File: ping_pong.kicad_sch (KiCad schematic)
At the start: 56 parts, among them J101 5V_IN, J102 AMMETER-, J103 GND_IN, J104 STEPPER_OUT1, J105 ENABLE, J106 STEP1, J107 DIR1, J108 AMMETER+, J109 STEP2, J110 DIR2, J111 STEPPER_OUT2, J112 12V_IN, J113 STEP3, J114 DIR3, J115 STEPPER_OUT3, J117 STEP4, J118 DIR4, J119 STEPPER_OUT4, J120 6V_for_Hbridge, J121 5V_for_ultrasonic1, J122 5V_for_ultrasonic2, J123 5V_for_ultrasonic3, J124 5V_for_ultrasonic4, J125 GND_for_ultrasonic1, J126 GND_for_ultrasonic2, J127 GND_for_ultrasonic3, J128 GND_for_ultrasonic4, J129 5V_for_pixycam, J130 GND_for_Hbridge, J131 3.3V_IN, J132 GND_for_xbee, J133 GND_for_pixycam, J134 GND_backup1, J135 GND_backup2, J138 5V_backup1, J139 5V_backup2, J140 5V_backup3, J141 5V_backup4, J142 3.3V_for_xbee, J143 3.3V_backup1, J144 3.3V_backup2, J145 5V_SERVO1, J146 5V_SERVO2, J147 GND_SERVO1, J148 GND_SERVO1

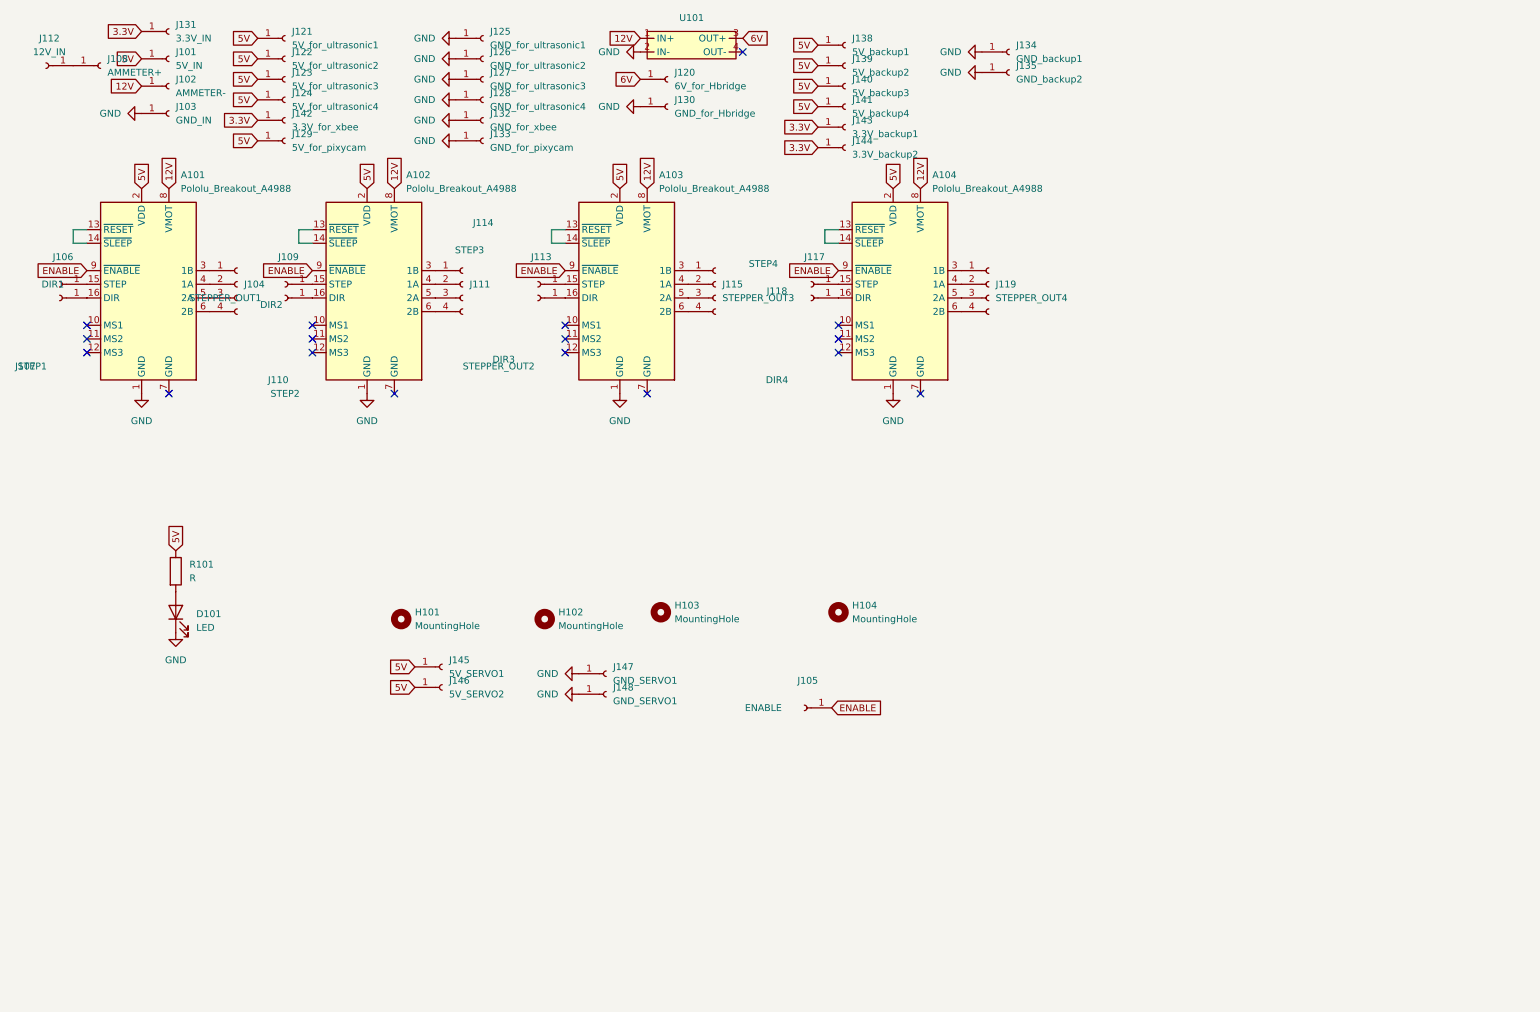
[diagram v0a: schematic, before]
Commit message: checkpoint
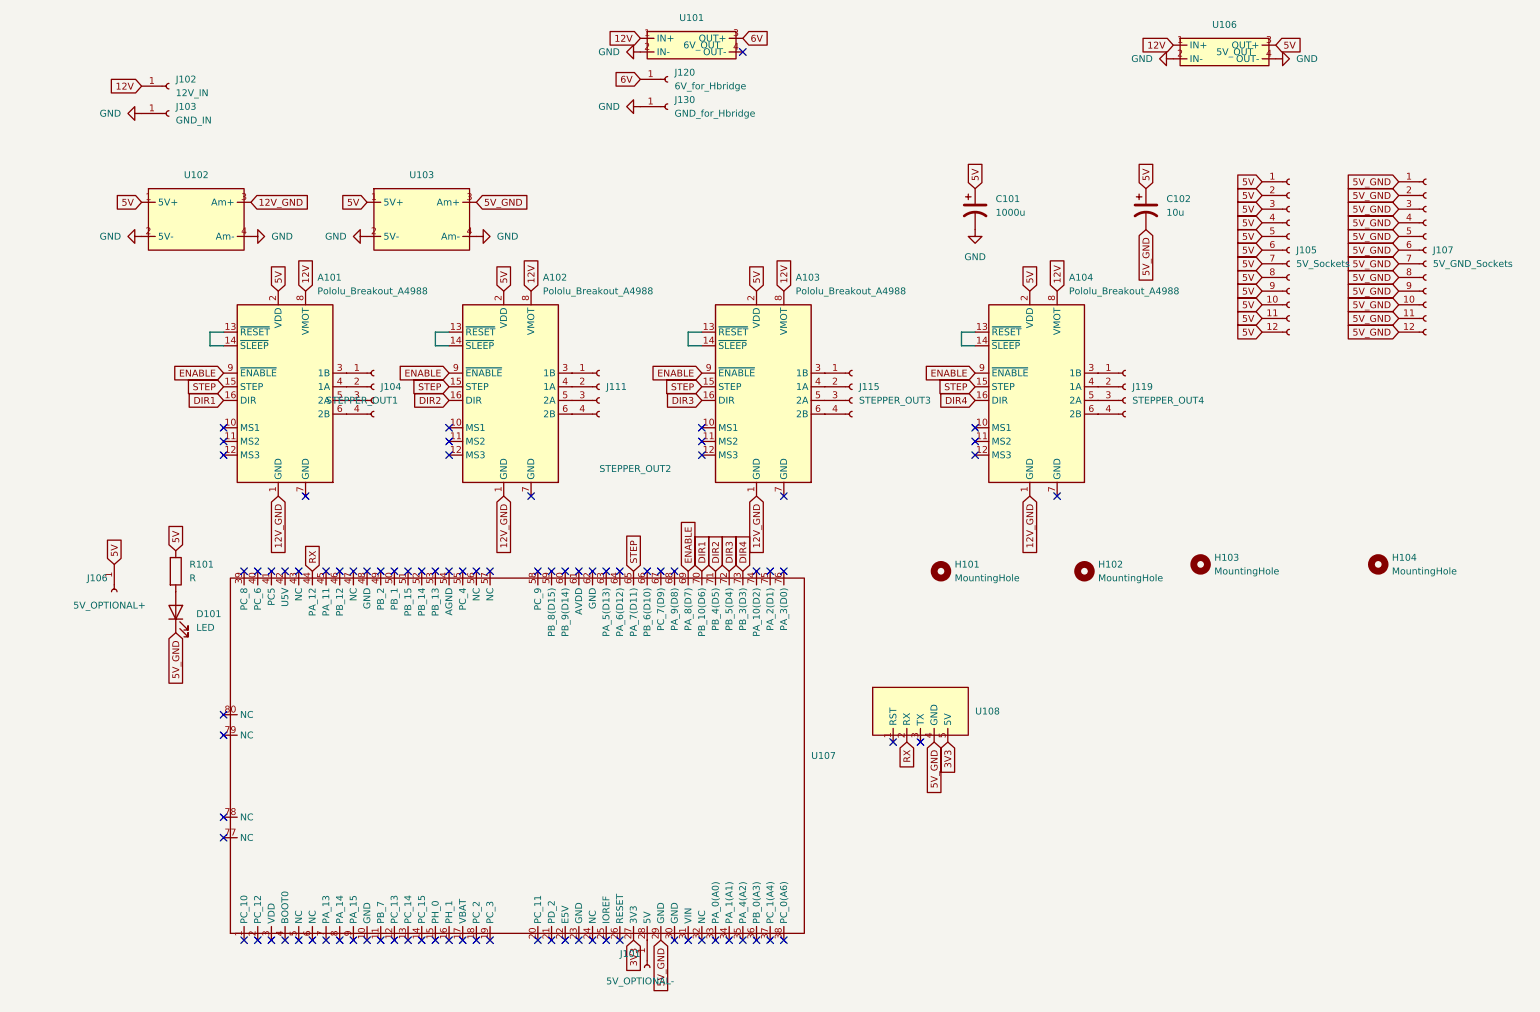
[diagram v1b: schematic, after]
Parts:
- removed J105: ENABLE, MyPinSocket:MyPinSocket, symbol Connector:Conn_01x01_Socket
- removed J107: DIR1, MyPinSocket:MyPinSocket, symbol Connector:Conn_01x01_Socket
- removed J108: AMMETER+, MyPinSocket:MyPinSocket, symbol Connector:Conn_01x01_Socket
- removed J109: STEP2, MyPinSocket:MyPinSocket, symbol Connector:Conn_01x01_Socket
- removed J110: DIR2, MyPinSocket:MyPinSocket, symbol Connector:Conn_01x01_Socket
- removed J112: 12V_IN, MyPinSocket:MyPinSocket, symbol Connector:Conn_01x01_Socket
- removed J113: STEP3, MyPinSocket:MyPinSocket, symbol Connector:Conn_01x01_Socket
- removed J114: DIR3, MyPinSocket:MyPinSocket, symbol Connector:Conn_01x01_Socket
- removed J117: STEP4, MyPinSocket:MyPinSocket, symbol Connector:Conn_01x01_Socket
- removed J118: DIR4, MyPinSocket:MyPinSocket, symbol Connector:Conn_01x01_Socket
- removed J121: 5V_for_ultrasonic1, MyPinSocket:MyPinSocket, symbol Connector:Conn_01x01_Socket
- removed J122: 5V_for_ultrasonic2, MyPinSocket:MyPinSocket, symbol Connector:Conn_01x01_Socket
- removed J123: 5V_for_ultrasonic3, MyPinSocket:MyPinSocket, symbol Connector:Conn_01x01_Socket
- removed J124: 5V_for_ultrasonic4, MyPinSocket:MyPinSocket, symbol Connector:Conn_01x01_Socket
- removed J125: GND_for_ultrasonic1, MyPinSocket:MyPinSocket, symbol Connector:Conn_01x01_Socket
- removed J126: GND_for_ultrasonic2, MyPinSocket:MyPinSocket, symbol Connector:Conn_01x01_Socket
- removed J127: GND_for_ultrasonic3, MyPinSocket:MyPinSocket, symbol Connector:Conn_01x01_Socket
- removed J128: GND_for_ultrasonic4, MyPinSocket:MyPinSocket, symbol Connector:Conn_01x01_Socket
- removed J129: 5V_for_pixycam, MyPinSocket:MyPinSocket, symbol Connector:Conn_01x01_Socket
- removed J131: 3.3V_IN, MyPinSocket:MyPinSocket, symbol Connector:Conn_01x01_Socket
- removed J132: GND_for_xbee, MyPinSocket:MyPinSocket, symbol Connector:Conn_01x01_Socket
- removed J133: GND_for_pixycam, MyPinSocket:MyPinSocket, symbol Connector:Conn_01x01_Socket
- removed J134: GND_backup1, MyPinSocket:MyPinSocket, symbol Connector:Conn_01x01_Socket
- removed J135: GND_backup2, MyPinSocket:MyPinSocket, symbol Connector:Conn_01x01_Socket
- removed J138: 5V_backup1, MyPinSocket:MyPinSocket, symbol Connector:Conn_01x01_Socket
- removed J139: 5V_backup2, MyPinSocket:MyPinSocket, symbol Connector:Conn_01x01_Socket
- removed J140: 5V_backup3, MyPinSocket:MyPinSocket, symbol Connector:Conn_01x01_Socket
- removed J141: 5V_backup4, MyPinSocket:MyPinSocket, symbol Connector:Conn_01x01_Socket
- removed J142: 3.3V_for_xbee, MyPinSocket:MyPinSocket, symbol Connector:Conn_01x01_Socket
- removed J143: 3.3V_backup1, MyPinSocket:MyPinSocket, symbol Connector:Conn_01x01_Socket
- removed J144: 3.3V_backup2, MyPinSocket:MyPinSocket, symbol Connector:Conn_01x01_Socket
- removed J145: 5V_SERVO1, MyPinSocket:MyPinSocket, symbol Connector:Conn_01x01_Socket
- removed J146: 5V_SERVO2, MyPinSocket:MyPinSocket, symbol Connector:Conn_01x01_Socket
- removed J147, J148: GND_SERVO1, MyPinSocket:MyPinSocket, symbol Connector:Conn_01x01_Socket
- added C101: 1000u, Capacitor_THT:CP_Radial_D10.0mm_P5.00mm, symbol Device:C_Polarized_US
- added C102: 10u, Capacitor_THT:CP_Radial_D5.0mm_P2.00mm, symbol Device:C_Polarized_US
- added J105: 5V_Sockets, Connector_PinSocket_2.54mm:PinSocket_1x12_P2.54mm_Vertical, symbol Connector:Conn_01x12_Socket
- added J107: 5V_GND_Sockets, Connector_PinSocket_2.54mm:PinSocket_1x12_P2.54mm_Vertical, symbol Connector:Conn_01x12_Socket
- added U102, U103: ~, Ammeter:Ammeter, symbol MyAmmeter:MyAmmeter
- added U106: 5V_OUT, LM2596:LM2596, symbol LM2596:LM2596
- added U107: ~, NUCLEO-F401RE:NUCLEO-F401RE, symbol NUCLEO-F401RE:NUCLEO-F401RE
- added U108: ~, XBEE:XBEE, symbol XBEE:XBEE
- J101: value 5V_IN -> 5V_OPTIONAL-
- J102: value AMMETER- -> 12V_IN
- J106: value STEP1 -> 5V_OPTIONAL+
- U101: value ~ -> 6V_OUT
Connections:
- net 12V: now also U106.1 (IN+)
- net 5V: now also J106.1 (Pin_1), C101.1, C102.1, J105.1 (Pin_1), J105.10 (Pin_10), J105.11 (Pin_11), J105.12 (Pin_12), J105.2 (Pin_2), J105.3 (Pin_3), J105.4 (Pin_4), J105.5 (Pin_5), J105.6 (Pin_6), J105.7 (Pin_7), J105.8 (Pin_8), J105.9 (Pin_9), U102.1 (5V+), U103.1 (5V+), U106.3 (OUT+); no longer J101.1 (Pin_1)
- net ENABLE: now also U107.69 (PA_8(D7))
- net GND: now also C101.2, U102.2 (5V-), U102.4 (Am-), U103.2 (5V-), U103.4 (Am-), U106.2 (IN-), U106.4 (OUT-); no longer A101.1 (GND), A102.1 (GND), A103.1 (GND), A104.1 (GND), D101.1 (K)
- net DIR3: now reaches A103.16 (DIR)
- net DIR3: now also U107.72 (PB_5(D4))
- net STEP: now reaches A104.15 (STEP)
- net STEP: now also A101.15 (STEP), A102.15 (STEP), A103.15 (STEP), U107.65 (PA_7(D11))
- net DIR2: now reaches A102.16 (DIR)
- net DIR2: now also U107.71 (PB_4(D5))
- net DIR1: now reaches A101.16 (DIR)
- net DIR1: now also U107.70 (PB_10(D6))
- net DIR4: now reaches A104.16 (DIR)
- net DIR4: now also U107.73 (PB_3(D3))
- new net: J101.1 (Pin_1), U107.28 (5V)
- new net 12V_GND: A101.1 (GND), A102.1 (GND), A103.1 (GND), A104.1 (GND), U102.3 (Am+)
- new net 3V3: U107.27 (3V3), U108.5 (5V)
- new net 5V_GND: C102.2, D101.1 (K), J107.1 (Pin_1), J107.10 (Pin_10), J107.11 (Pin_11), J107.12 (Pin_12), J107.2 (Pin_2), J107.3 (Pin_3), J107.4 (Pin_4), J107.5 (Pin_5), J107.6 (Pin_6), J107.7 (Pin_7), J107.8 (Pin_8), J107.9 (Pin_9), U103.3 (Am+), U107.29 (GND), U108.4 (GND)
- new net RX: U107.44 (PA_12), U108.2 (RX)
- no-connect marks 17 -> 89
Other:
- moved on the sheet: A101, A102, A103, A104, H101, H102, H103, H104, J104, J111, J115, J119

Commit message: checkpoint
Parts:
- C102: footprint Capacitor_THT:CP_Radial_D5.0mm_P2.00mm -> Capacitor_THT:CP_Radial_D5.0mm_P2.50mm
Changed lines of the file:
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@@
       (effects (font (size 1.27 1.27)) (justify left))
     )
-    (property "Footprint" "Capacitor_THT:CP_Radial_D5.0mm_P2.00mm" (at 219.71 50.8 0)
+    (property "Footprint" "Capacitor_THT:CP_Radial_D5.0mm_P2.50mm" (at 219.71 50.8 0)
       (effects (font (size 1.27 1.27)) hide)
     )
